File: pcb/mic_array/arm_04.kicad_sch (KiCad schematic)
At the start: 16 parts, among them U33 IM72D128V01XTMA1, U34 IM72D128V01XTMA1, U35 IM72D128V01XTMA1, U36 IM72D128V01XTMA1, U37 IM72D128V01XTMA1, U38 IM72D128V01XTMA1, U39 IM72D128V01XTMA1, U40 IM72D128V01XTMA1

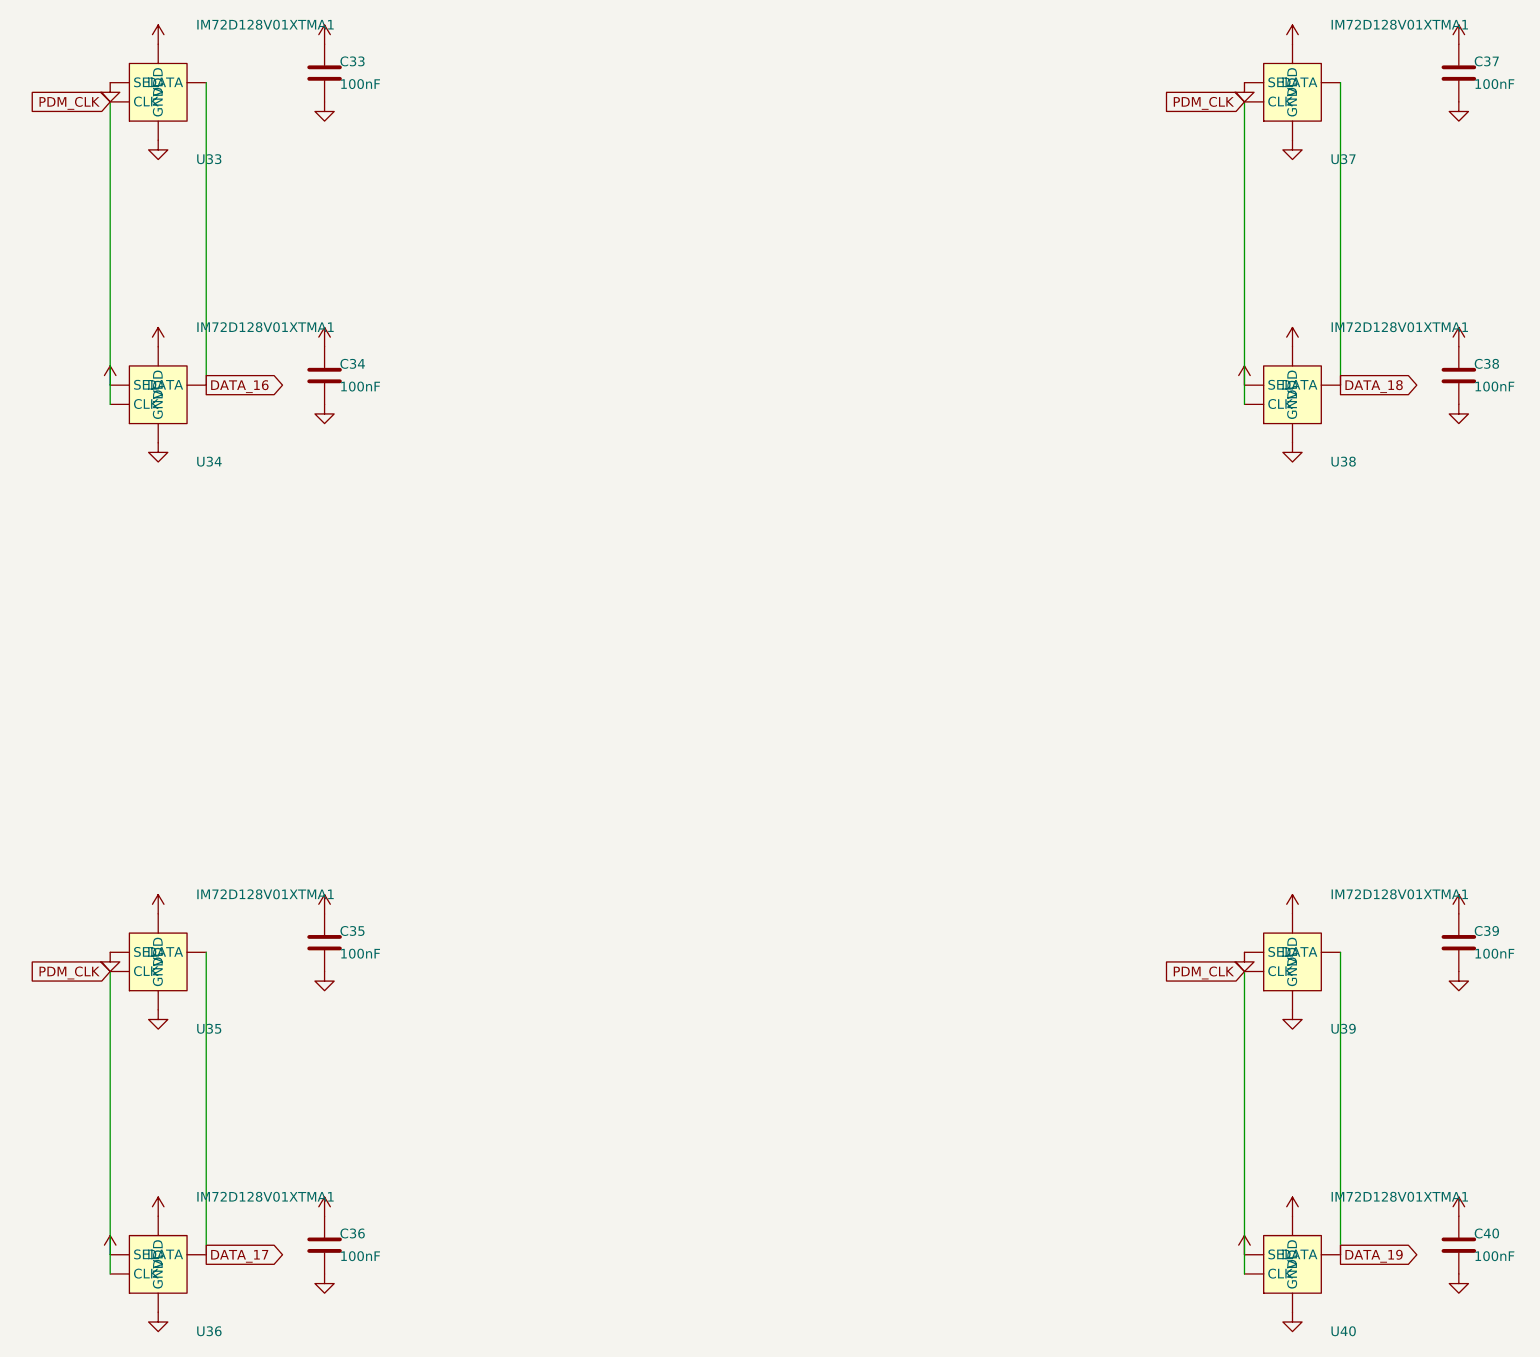
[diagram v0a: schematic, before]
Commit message: Updated.
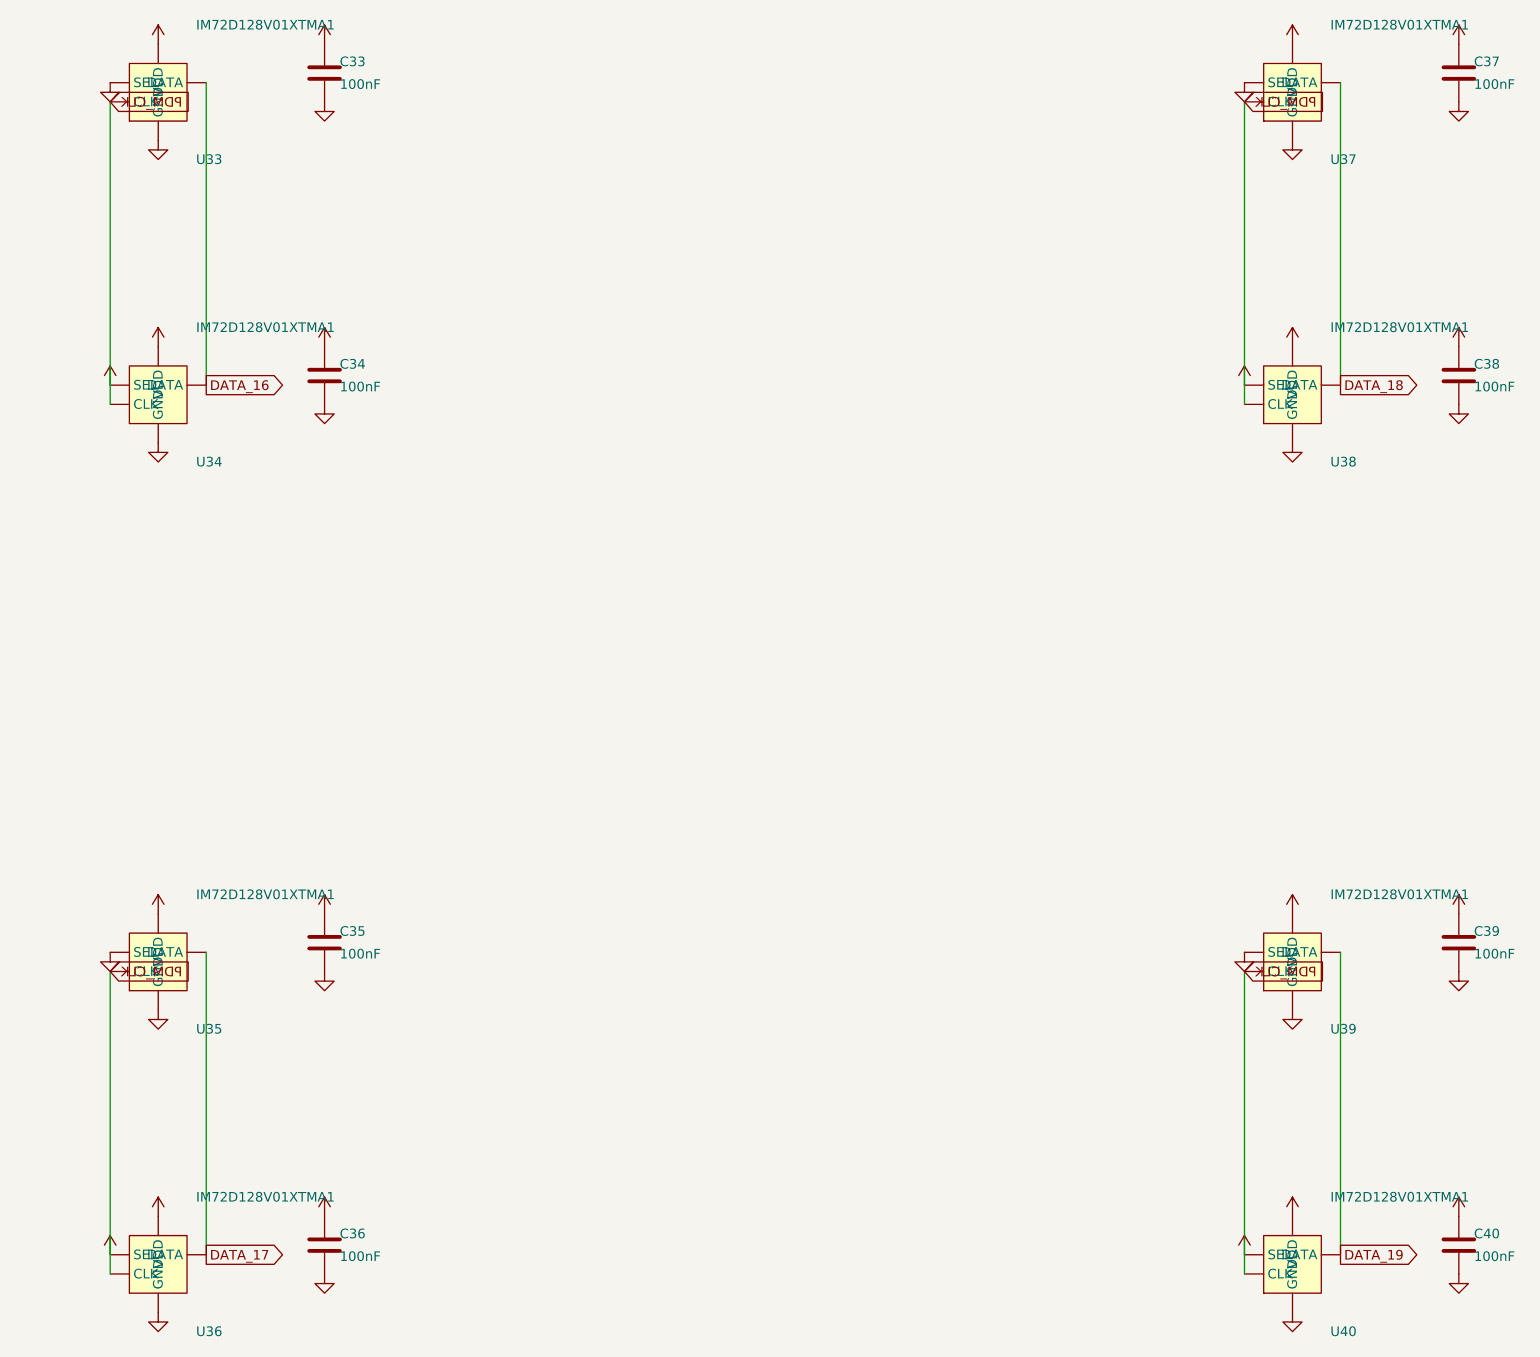
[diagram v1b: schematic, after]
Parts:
- C33, C34, C35, C36, C37, C38, C39, C40: footprint Capacitor_SMD:C_0402_1005Metric -> (none)
- U33, U34, U35, U36, U37, U38, U39, U40: footprint Sensor_Audio:Infineon_PG-LLGA-5-2 -> (none)
